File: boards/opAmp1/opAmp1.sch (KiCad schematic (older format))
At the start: 31 parts, among them P1 CONN_01X02, P2 CONN_01X02, P3 CONN_01X02, Q1 TIP122, Q2 BC817-40

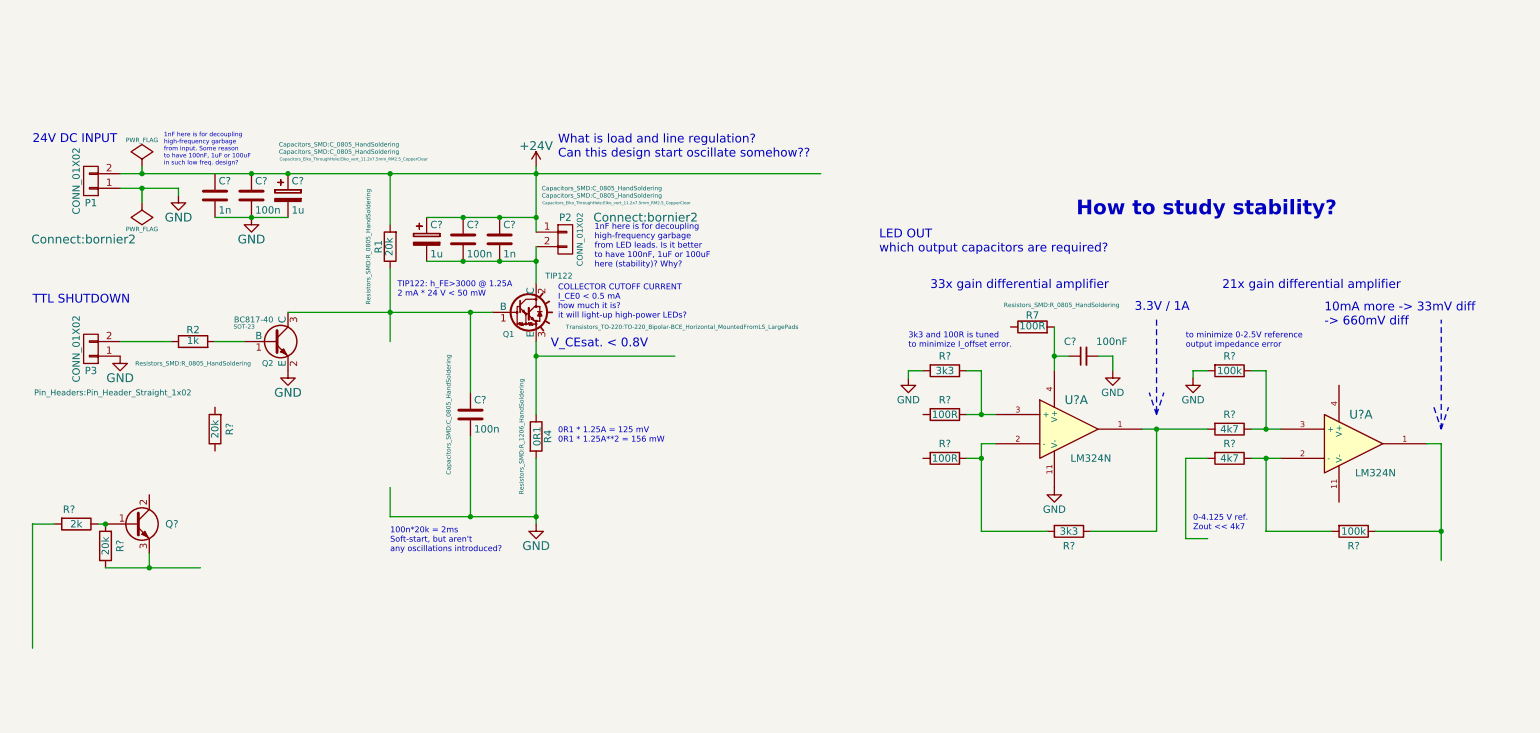
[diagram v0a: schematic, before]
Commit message: upgrade
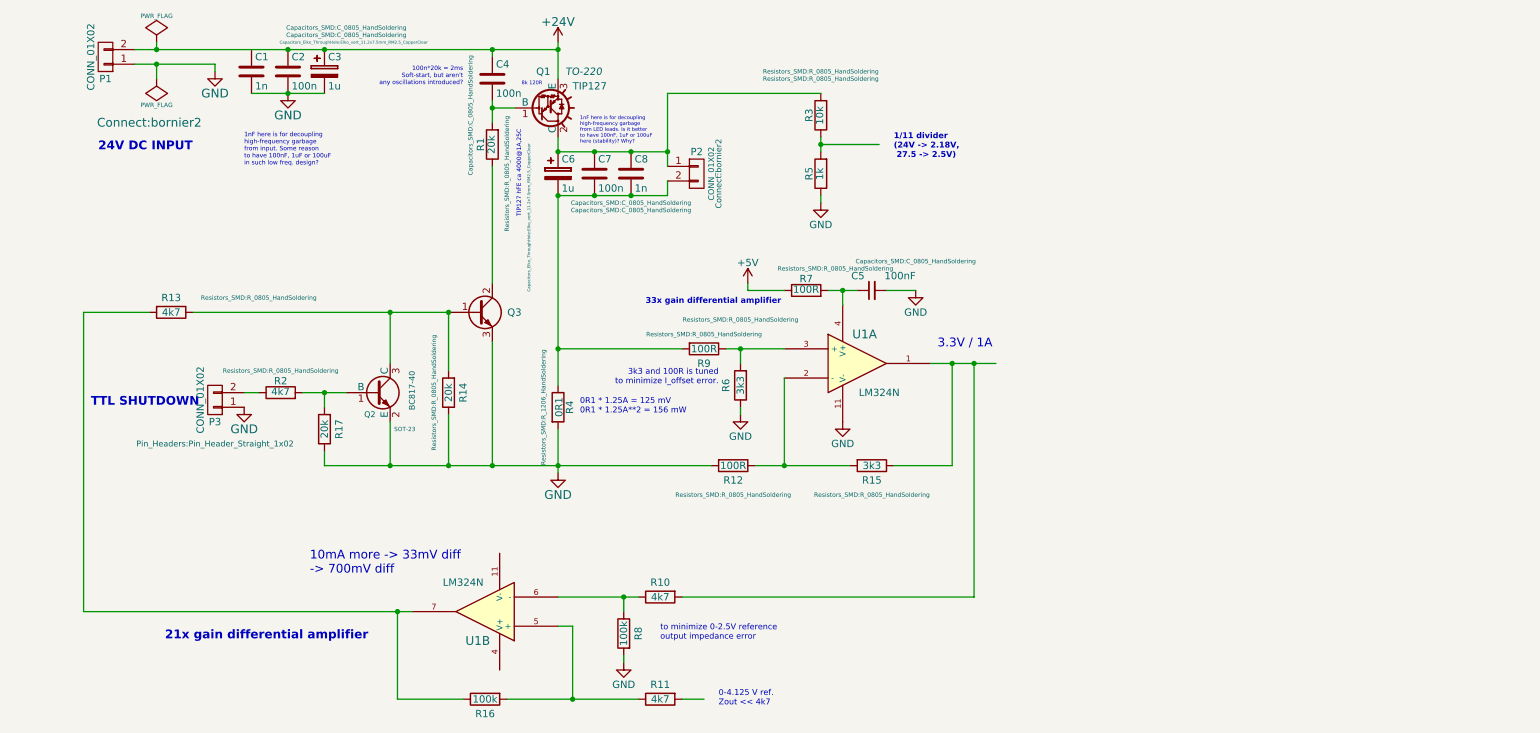
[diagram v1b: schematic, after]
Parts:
- removed Q1: TIP122, Transistors_TO-220:TO-220_Bipolar-BCE_Horizontal_MountedFromLS_LargePads, symbol TIP122
- removed R?: 20k, symbol R
- added Q1: TIP127, TO-220, symbol TIP127
- added R17: 20k, symbol R
- added R3: 10k, Resistors_SMD:R_0805_HandSoldering, symbol R
- added R5: 1k, Resistors_SMD:R_0805_HandSoldering, symbol R
- C5: renamed from C?; footprint (none) -> Capacitors_SMD:C_0805_HandSoldering
- R12, R14, R15, R6, R9: renamed from R?; footprint (none) -> Resistors_SMD:R_0805_HandSoldering
- R13: renamed from R?; value 2k -> 4k7; footprint (none) -> Resistors_SMD:R_0805_HandSoldering
- R2: value 1k -> 4k7
- gave numbers to parts that had none: 13
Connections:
- net labels added: +5V
- wire segments 65 -> 92
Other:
- note added: "1/11 divider\n(24V -> 2.18V,\n 27.5 -> 2.5V)"
- note added: "10mA more -> 33mV diff\n-> 700mV diff"
- note added: "8k 120R"
- note added: "TIP127 hFE ca 4000@1A,25C"
- note removed: "10mA more -> 33mV diff\n-> 660mV diff"
- note removed: "COLLECTOR CUTOFF CURRENT\nI_CE0 < 0.5 mA\nhow much it is?\nit will light-up high-power LEDs?"
- note removed: "How to study stability?"
- note removed: "LED OUT\nwhich output capacitors are required?"
- note removed: "TIP122: h_FE>3000 @ 1.25A\n2 mA * 24 V < 50 mW"
- note removed: "V_CEsat. < 0.8V"
- note removed: "What is load and line regulation?\nCan this design start oscillate somehow??"
- moved on the sheet: C1, C2, C3, C4, C5, C6, C7, C8, P1, P2, P3, Q2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
